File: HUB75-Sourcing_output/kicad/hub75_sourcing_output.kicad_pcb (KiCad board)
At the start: 2 copper layers, 85 x 56 mm, 128 parts, among them J1 Conn_01x02_Male, J10 Conn_01x02_Male, J11 Conn_01x02_Male, J12 Conn_01x02_Male, J13 Screw_Terminal_01x02, J2 Conn_01x02_Male, J3 Conn_01x02_Male, J4 Conn_01x02_Male, J5 Conn_01x02_Male, J6 Conn_01x02_Male, J7 Conn_01x02_Male, J8 Conn_01x02_Male, J9 Conn_01x02_Male, Q1 BSS84, Q10 BSS84, Q11 BSS84, Q12 BSS84, Q13 AO3401A, Q14 2N7002, Q15 2N7002, Q16 2N7002, Q17 2N7002, Q18 2N7002, Q19 2N7002, Q2 BSS84, Q20 2N7002, Q21 2N7002, Q22 2N7002, Q23 2N7002, Q24 2N7002, Q25 2N7002, Q26 2N7002, Q3 BSS84, Q4 BSS84, Q5 BSS84, Q6 BSS84, Q7 BSS84, Q8 BSS84, Q9 BSS84, U1 LTV-827, U10 LTV-827, U13 LTV-827, U16 LTV-827, U2 HV9921N8-G, U4 LTV-827, U7 LTV-827

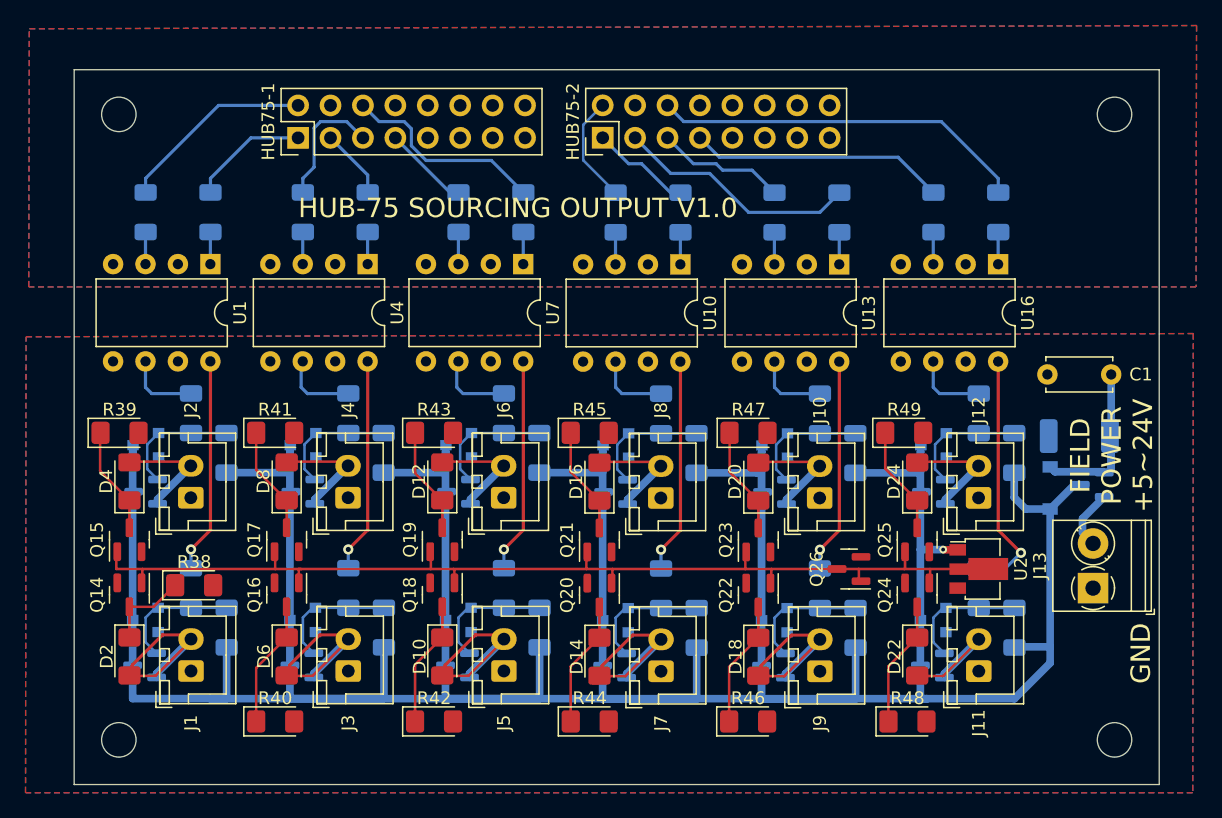
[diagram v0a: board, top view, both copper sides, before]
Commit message: Update label
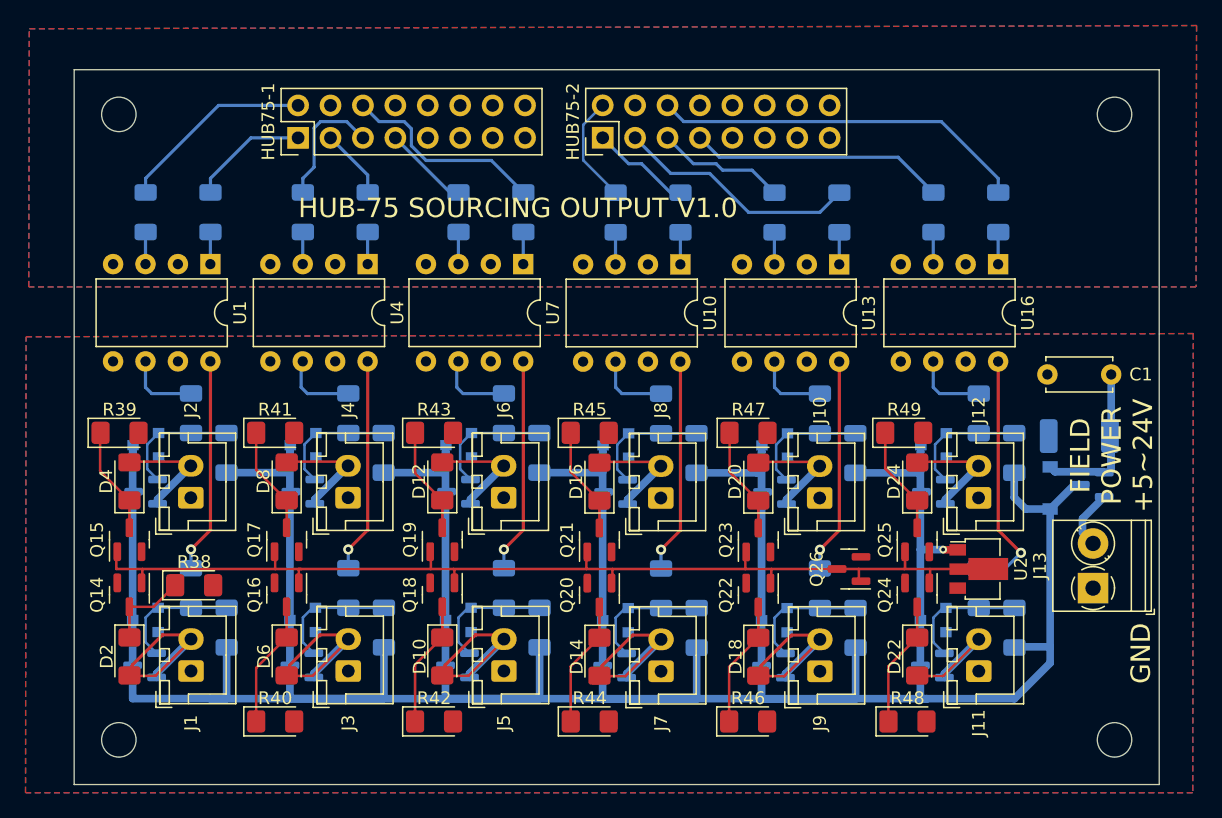
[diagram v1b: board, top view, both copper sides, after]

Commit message: Regenerated
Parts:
- U2: value HV9921N8-G -> CL2N8-G
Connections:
- HUB75-1 pad 8: GND -> unconnected-(HUB75-1-Pad8)
- HUB75-2 pad 8: GND -> unconnected-(HUB75-2-Pad8)
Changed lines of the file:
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@@
   (net 97 "Net-(D1-Pad2)")
   (net 98 "CUR_MIRROR")
+  (net 99 "unconnected-(HUB75-1-Pad8)")
+  (net 100 "unconnected-(HUB75-2-Pad8)")
   (footprint "Connector_JST:JST_XH_B2B-XH-A_1x02_P2.50mm_Vertical" (layer "F.Cu")
     (at 109.474 97.673 90)
@@
     (property "Sheetfile" "FET-driver.kicad_sch")
     (property "Sheetname" "FET-driver1")
+    (property "exclude_from_bom" "")
     (attr smd exclude_from_pos_files exclude_from_bom)
     (fp_text reference "R40" (at 0 -1.82) (layer "F.SilkS")
@@
     (property "Sheetfile" "FET-driver.kicad_sch")
     (property "Sheetname" "FET-driver2")
+    (property "exclude_from_bom" "")
     (attr smd exclude_from_pos_files exclude_from_bom)
     (fp_text reference "R39" (at 0 -1.82) (layer "F.SilkS")
@@
     (property "Sheetfile" "FET-driver.kicad_sch")
     (property "Sheetname" "FET-driver1")
+    (property "exclude_from_bom" "")
     (attr smd exclude_from_pos_files exclude_from_bom)
     (fp_text reference "R38" (at 0 -1.82) (layer "F.SilkS")
@@
     (property "Sheetfile" "FET-driver.kicad_sch")
     (property "Sheetname" "FET-driver2")
+    (property "exclude_from_bom" "")
     (attr smd exclude_from_pos_files exclude_from_bom)
     (fp_text reference "R47" (at 0 -1.82) (layer "F.SilkS")
@@
     (property "Sheetfile" "FET-driver.kicad_sch")
     (property "Sheetname" "FET-driver1")
+    (property "exclude_from_bom" "")
     (attr smd exclude_from_pos_files exclude_from_bom)
     (fp_text reference "R48" (at 0 -1.82) (layer "F.SilkS")
@@
     (property "Sheetfile" "FET-driver.kicad_sch")
     (property "Sheetname" "FET-driver2")
+    (property "exclude_from_bom" "")
     (attr smd exclude_from_pos_files exclude_from_bom)
     (fp_text reference "R41" (at 0 -1.82) (layer "F.SilkS")
@@
       (net 16 "GPIO1-6") (pinfunction "Pin_7") (pintype "passive"))
     (pad "8" thru_hole oval (at 2.54 7.62 90) (size 1.7 1.7) (drill 1) (layers *.Cu *.Mask)
-      (net 4 "GND") (pinfunction "Pin_8") (pintype "passive"))
+      (net 99 "unconnected-(HUB75-1-Pad8)") (pinfunction "Pin_8") (pintype "passive"))
     (pad "9" thru_hole oval (at 0 10.16 90) (size 1.7 1.7) (drill 1) (layers *.Cu *.Mask)
       (net 61 "unconnected-(HUB75-1-Pad9)") (pinfunction "Pin_9") (pintype "passive"))
@@
     (property "Sheetfile" "FET-driver.kicad_sch")
     (property "Sheetname" "FET-driver2")
+    (property "exclude_from_bom" "")
     (attr smd exclude_from_pos_files exclude_from_bom)
     (fp_text reference "R49" (at 0 -1.82) (layer "F.SilkS")
@@
       (effects (font (size 1 1) (thickness 0.15)))
     )
-    (fp_text value "HV9921N8-G" (at 0.3 3.5) (layer "F.Fab") hide
+    (fp_text value "CL2N8-G" (at 0.3 3.5) (layer "F.Fab") hide
       (effects (font (size 1 1) (thickness 0.15)))
     )
@@
       (net 26 "GPIO2-6") (pinfunction "Pin_7") (pintype "passive"))
     (pad "8" thru_hole oval (at 2.54 7.62 90) (size 1.7 1.7) (drill 1) (layers *.Cu *.Mask)
-      (net 4 "GND") (pinfunction "Pin_8") (pintype "passive"))
+      (net 100 "unconnected-(HUB75-2-Pad8)") (pinfunction "Pin_8") (pintype "passive"))
     (pad "9" thru_hole oval (at 0 10.16 90) (size 1.7 1.7) (drill 1) (layers *.Cu *.Mask)
       (net 47 "unconnected-(HUB75-2-Pad9)") (pinfunction "Pin_9") (pintype "passive"))
@@
     (property "Sheetfile" "FET-driver.kicad_sch")
     (property "Sheetname" "FET-driver1")
+    (property "exclude_from_bom" "")
     (attr smd exclude_from_pos_files exclude_from_bom)
     (fp_text reference "R44" (at 0 -1.82) (layer "F.SilkS")
@@
     (property "Sheetfile" "FET-driver.kicad_sch")
     (property "Sheetname" "FET-driver1")
+    (property "exclude_from_bom" "")
     (attr smd exclude_from_pos_files exclude_from_bom)
     (fp_text reference "R42" (at 0 -1.82) (layer "F.SilkS")
@@
     (property "Sheetfile" "FET-driver.kicad_sch")
     (property "Sheetname" "FET-driver2")
+    (property "exclude_from_bom" "")
     (attr smd exclude_from_pos_files exclude_from_bom)
     (fp_text reference "R45" (at 0 -1.82) (layer "F.SilkS")
@@
     (property "Sheetfile" "FET-driver.kicad_sch")
     (property "Sheetname" "FET-driver2")
+    (property "exclude_from_bom" "")
     (attr smd exclude_from_pos_files exclude_from_bom)
     (fp_text reference "R43" (at 0 -1.82) (layer "F.SilkS")
@@
     (property "Sheetfile" "FET-driver.kicad_sch")
     (property "Sheetname" "FET-driver1")
+    (property "exclude_from_bom" "")
     (attr smd exclude_from_pos_files exclude_from_bom)
     (fp_text reference "R46" (at 0 -1.82) (layer "F.SilkS")
